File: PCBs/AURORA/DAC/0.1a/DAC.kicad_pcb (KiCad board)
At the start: 4 copper layers, 55 x 55.5 mm, 48 parts, among them J1 Conn_01x04_Pin, J11 Conn_01x02_Pin, J12 Conn_01x02_Pin, J2 Conn_01x03_Pin, J3 Conn_01x02_Pin, J4 Conn_01x03_Pin, J5 Conn_02x10_Odd_Even, J6 Conn_01x04_Pin, J7 Conn_01x03_Pin, J8 Conn_01x02_Pin, U1 ZLDO1117QG33TA, U2 PCM5142PWR

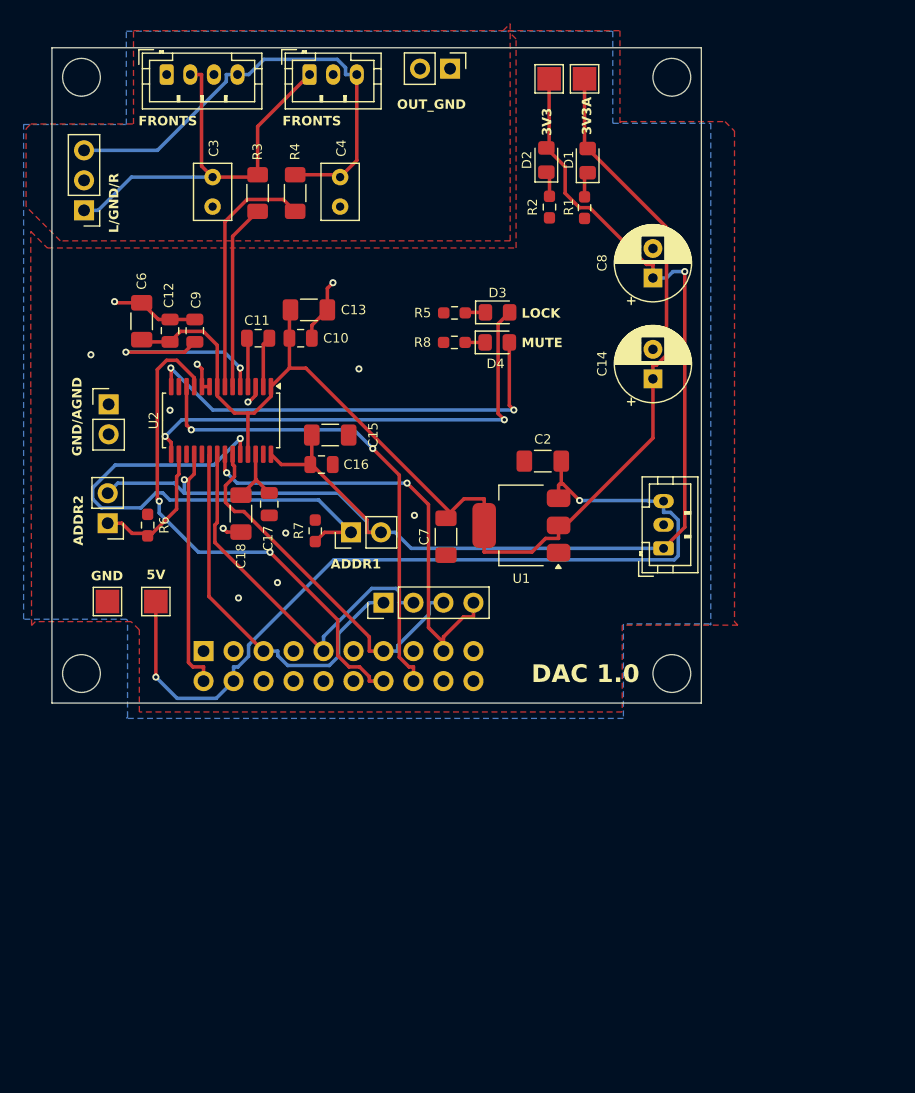
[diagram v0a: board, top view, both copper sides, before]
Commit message: Working?
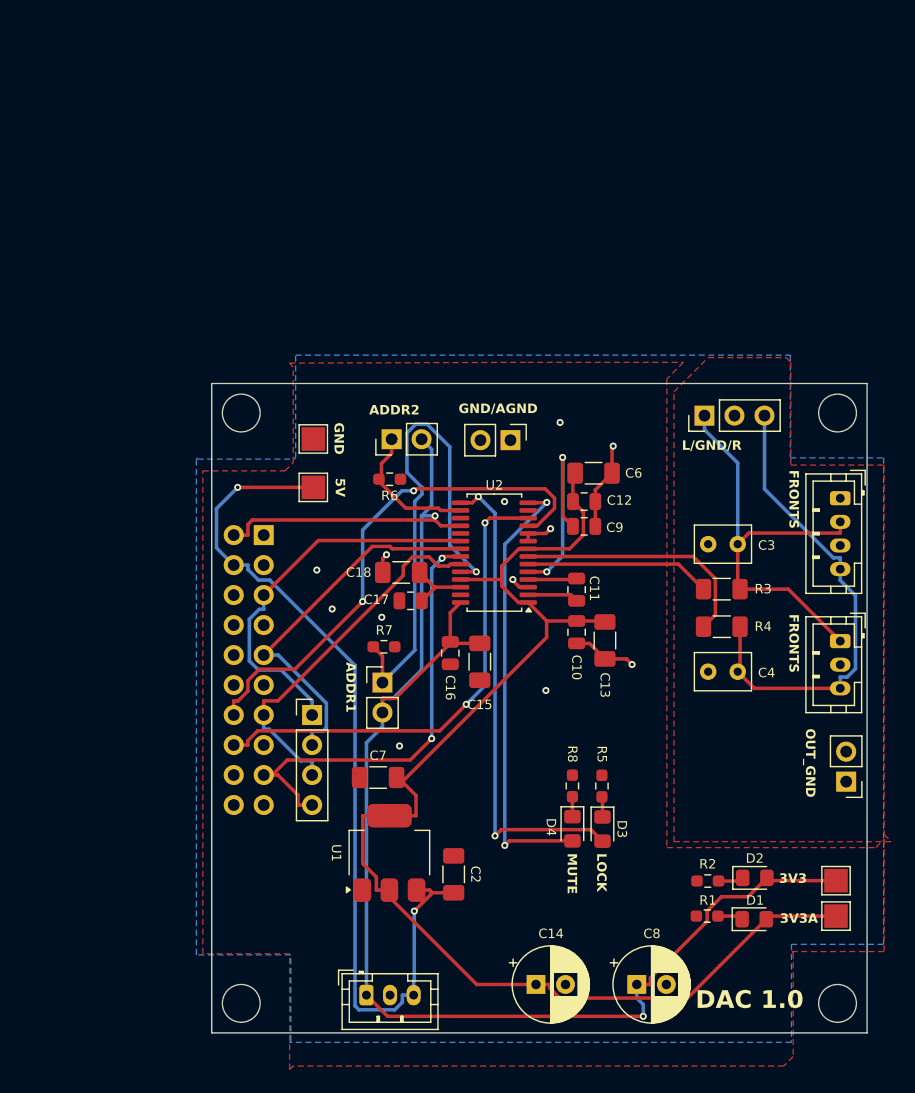
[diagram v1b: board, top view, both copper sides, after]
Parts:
- moved H2 79.7 mm to (109.0, 119.4), turned to -90 degrees
- moved TP1 74.0 mm to (108.9, 112.0), turned to 0 degrees
- moved TP3 72.1 mm to (108.9, 109.0), turned to 0 degrees
- moved H1 70.1 mm to (109.0, 69.4), turned to -90 degrees
- moved J3 69.1 mm to (109.8, 100.7), turned to 180 degrees
- moved J1 67.4 mm to (109.3, 76.7), turned to -90 degrees
- moved D1 65.8 mm to (102.0, 112.3), turned to 0 degrees
- moved J2 65.7 mm to (109.3, 88.8), turned to -90 degrees
- moved D2 63.3 mm to (102.0, 108.8), turned to 0 degrees
- moved R1 60.9 mm to (98.0, 112.0), turned to 0 degrees
- moved C8 59.9 mm to (92.0, 117.8), turned to 0 degrees
- moved R2 58.6 mm to (98.0, 109.1), turned to 0 degrees
- moved J4 55.3 mm to (97.8, 69.7), turned to 90 degrees
- moved C14 52.2 mm to (83.5, 117.8), turned to 0 degrees
- moved R3 51.7 mm to (99.2, 84.4), turned to 0 degrees
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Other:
- board size 55 x 55.5 mm -> 55.5 x 55 mm
